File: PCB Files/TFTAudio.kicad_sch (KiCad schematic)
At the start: 55 parts, among them J1 USB_C_Receptacle_USB2.0_14P, J2 Conn_01x02, J3 Conn_01x14_Socket, J5 Conn_01x12_Pin, Q1 BSS138, Q2 BSS138, Q3 DMG2301L, SW1 SW_SPST, U1 ESP32-WROVER-E, U2 CH340C, U3 MCP73831-2-OT, U4 AP2112K-3.3, U5 PCM5102A, X1 STEREO_AUDIO_JACK

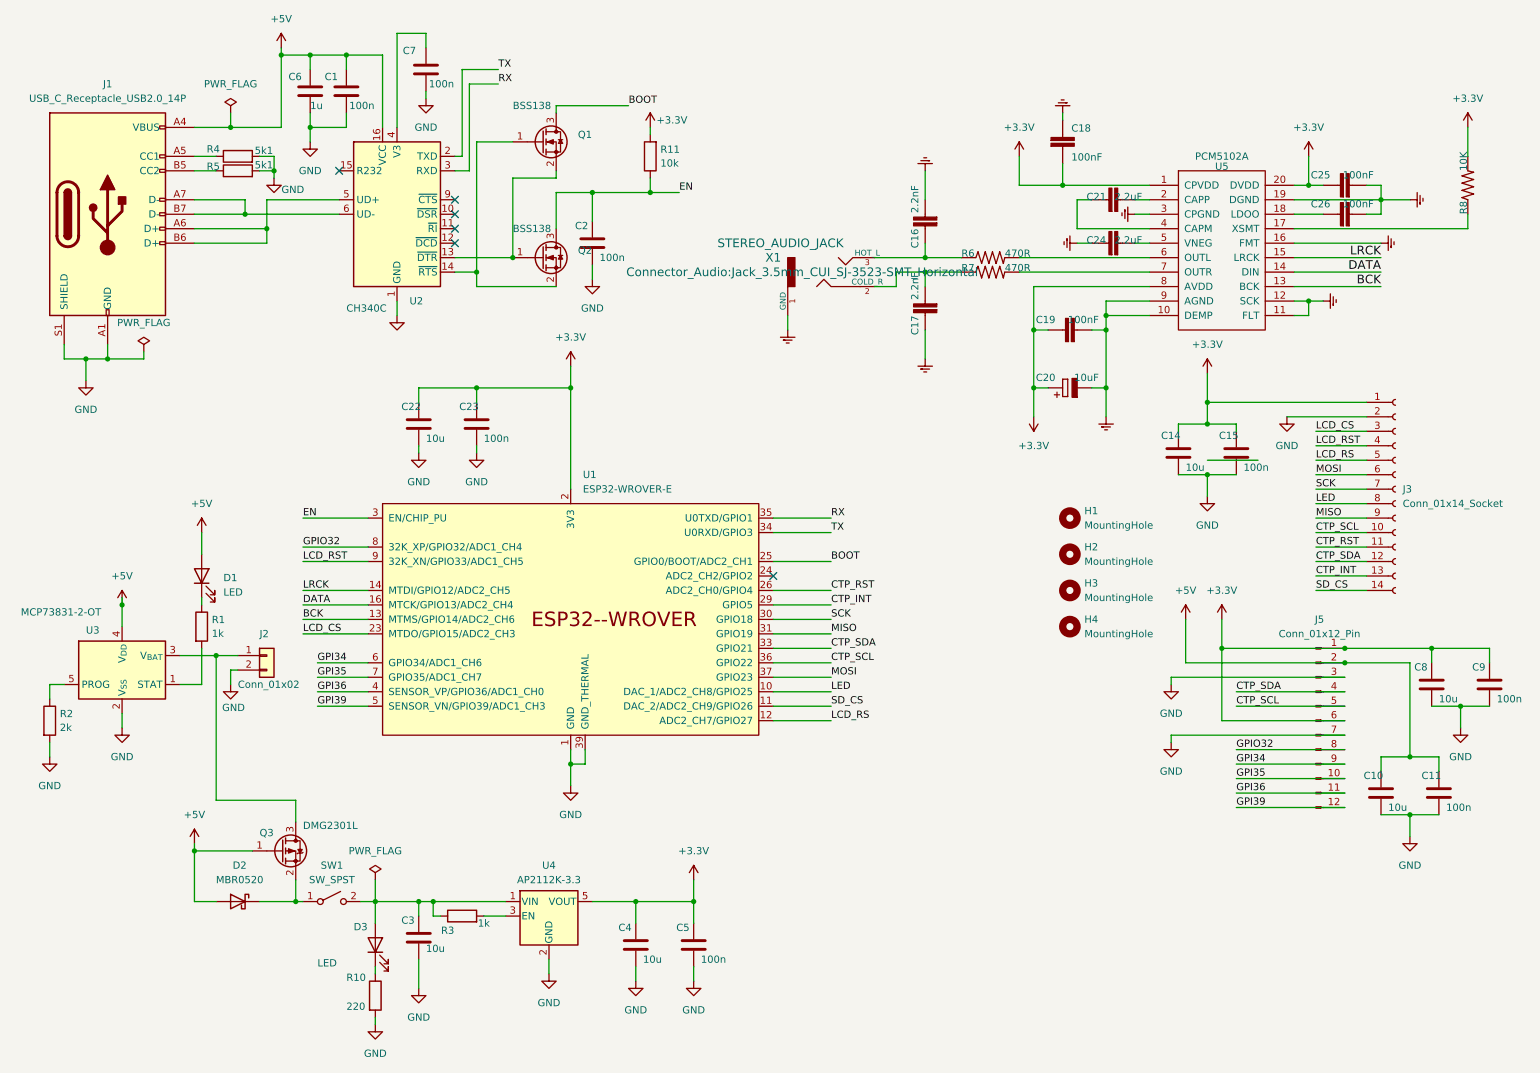
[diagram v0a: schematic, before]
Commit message: Mark R Commit - PCB help
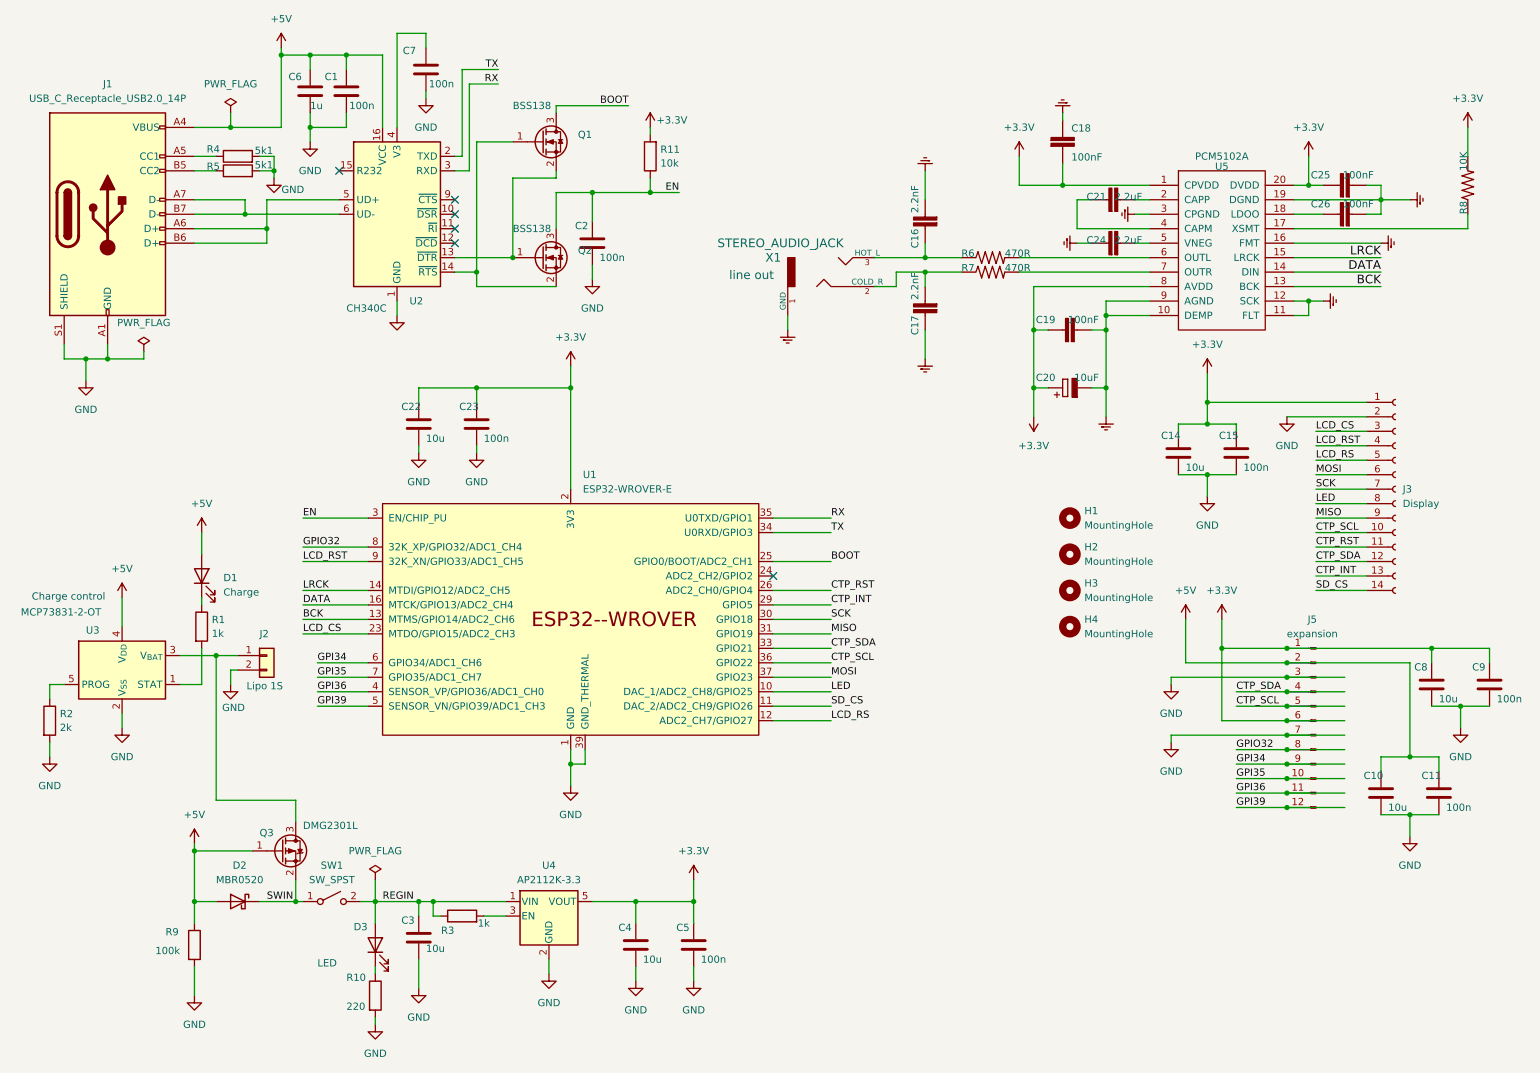
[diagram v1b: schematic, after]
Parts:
- added R9: 100k, Resistor_SMD:R_0603_1608Metric, symbol Device:R
- C10, C14, C22, C3, C4, C8: footprint Capacitor_SMD:C_0805_2012Metric_Pad1.18x1.45mm_HandSolder -> Capacitor_SMD:C_0603_1608Metric
- C17, C18, C19, C24, C25, C26: footprint Capacitor_SMD:C_0201_0603Metric -> Capacitor_SMD:C_0603_1608Metric
- C20, C21: footprint Capacitor_SMD:C_0805_2012Metric -> Capacitor_SMD:C_0603_1608Metric
- D1: value LED -> Charge
- H1, H2, H3, H4: footprint MountingHole:MountingHole_4.3mm_M4 -> MountingHole:MountingHole_3.2mm_M3_ISO14580
- J2: value Conn_01x02 -> Lipo 1S
- J3: value Conn_01x14_Socket -> Display
- J5: value Conn_01x12_Pin -> expansion
- X1: footprint Connector_Audio:Jack_3.5mm_CUI_SJ-3523-SMT_Horizontal -> line out
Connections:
- net +5V: now also R9.1
- net GND: now also R9.2
- net REGIN: now reaches C3.1, D3.2 (A), R3.1, SW1.2 (B), U4.1 (VIN)
- net SWIN: now reaches D2.1 (K), Q3.2 (S), SW1.1 (A)
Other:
- note added: "Charge control"
- moved on the sheet: J5
